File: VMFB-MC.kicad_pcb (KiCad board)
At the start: 2 copper layers, 64.6 x 67.3 mm, 45 parts, among them J1 Conn_01x04_Pin, J10 Conn_01x04_Pin, J2 Conn_01x04_Pin, J3 Conn_01x04_Pin, J4 Conn_01x02_Pin, J5 Conn_01x03_Pin, J6 Conn_01x04_Pin, J7 Conn_01x04_Pin, J8 Conn_01x04_Pin, J9 Conn_01x05_Pin, Q1 SFH313FA-2/3, Q2 SFH313FA-2/3, Q3 SFH313FA-2/3, Q4 SFH313FA-2/3, Q5 SFH313FA-2/3, Q6 SFH313FA-2/3, Q7 TIP120, Q8 TIP120, Q9 SFH313FA-2/3, U1 LM393

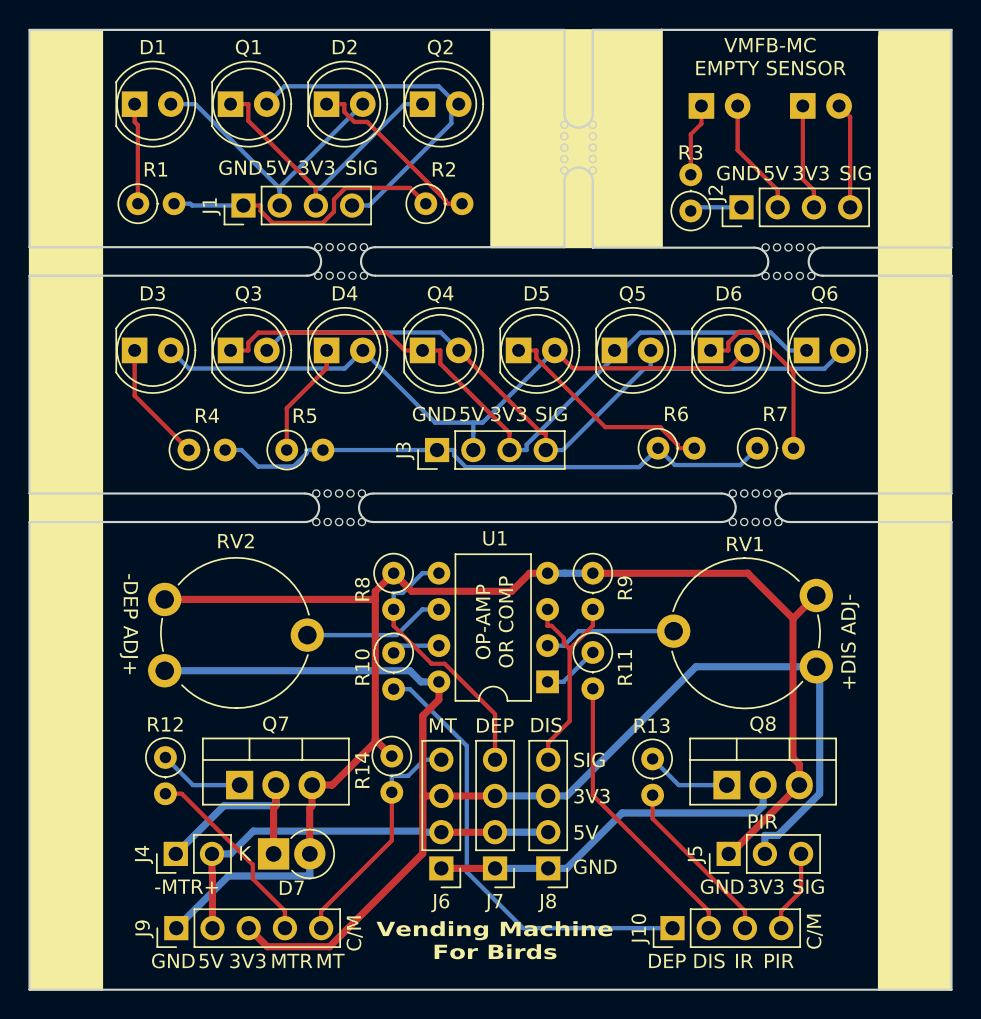
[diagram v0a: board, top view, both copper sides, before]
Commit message: more cleanup
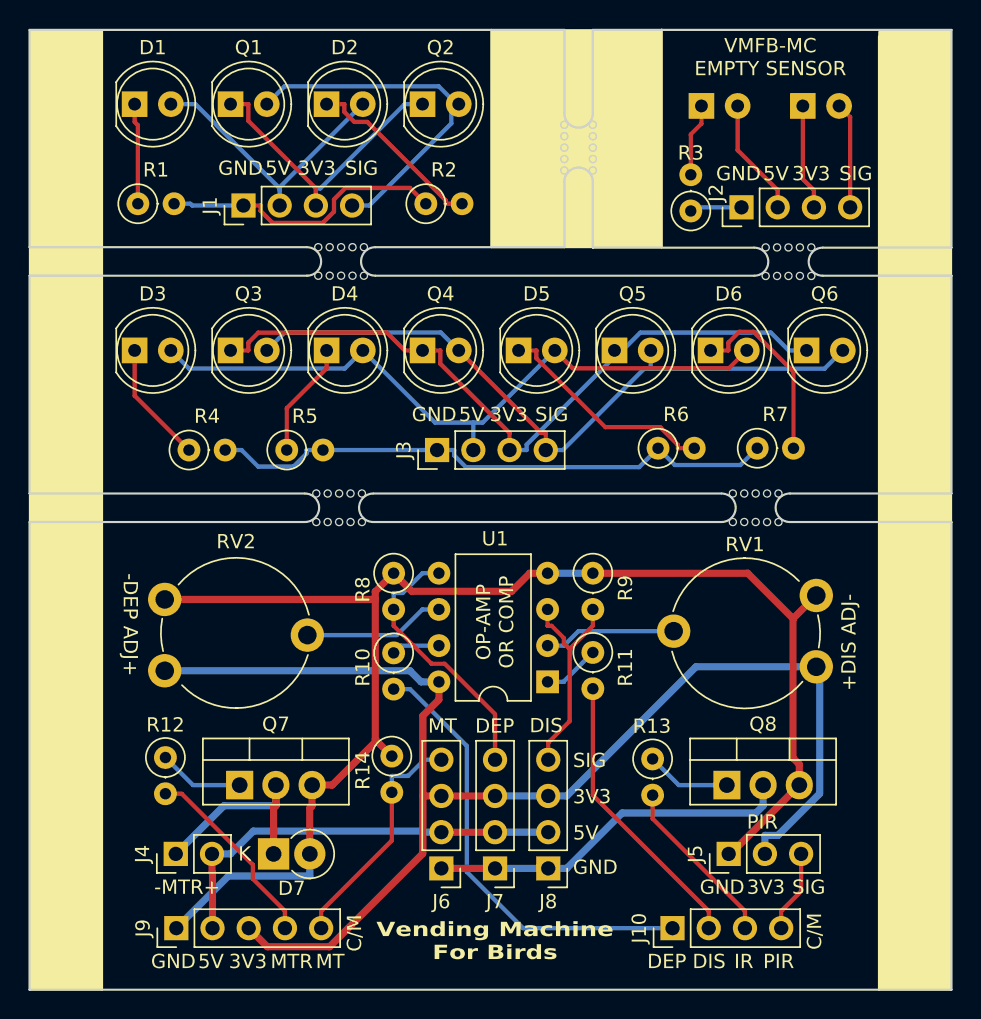
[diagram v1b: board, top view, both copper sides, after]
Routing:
- net Net-(J1-Pin_4): track 25.4 -> 24.5 mm
- net Net-(J3-Pin_3): track 50.6 -> 49.9 mm
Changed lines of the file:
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@@
   (segment (start 153.6182 101.1141) (end 153.6182 91.3248) (width 0.5) (layer "F.Cu") (net 2))
   (segment (start 133.8779 89.408) (end 126.873 89.408) (width 0.5) (layer "F.Cu") (net 2))
-  (segment (start 149.225 107.823) (end 149.098 107.823) (width 0.5) (layer "F.Cu") (net 2))
   (segment (start 154.051 101.5469) (end 153.6182 101.1141) (width 0.5) (layer "F.Cu") (net 2))
   (segment (start 119.888 104.4471) (end 119.726 104.6091) (width 0.5) (layer "F.Cu") (net 2))
@@
   (segment (start 119.726 107.823) (end 119.726 109.3731) (width 0.5) (layer "B.Cu") (net 2))
   (segment (start 114.0199 109.3731) (end 119.726 109.3731) (width 0.5) (layer "B.Cu") (net 2))
-  (segment (start 136.398 88.138) (end 137.6481 88.138) (width 0.5) (layer "B.Cu") (net 2))
+  (segment (start 136.398 88.138) (end 139.573 88.138) (width 0.5) (layer "B.Cu") (net 2))
   (segment (start 110.363 113.03) (end 114.0199 109.3731) (width 0.5) (layer "B.Cu") (net 2))
-  (segment (start 139.573 88.138) (end 137.6481 88.138) (width 0.5) (layer "B.Cu") (net 2))
   (segment (start 120.899 55.245) (end 122.1491 55.245) (width 0.3) (layer "F.Cu") (net 3))
   (segment (start 122.1491 55.792) (end 122.8522 56.4951) (width 0.3) (layer "F.Cu") (net 3))
@@
   (segment (start 132.715 103.759) (end 136.445 103.759) (width 0.5) (layer "B.Cu") (net 7))
   (segment (start 137.7451 103.759) (end 146.8021 94.702) (width 0.5) (layer "B.Cu") (net 7))
-  (segment (start 155.241 94.702) (end 155.478 94.939) (width 0.5) (layer "B.Cu") (net 7))
   (segment (start 151.638 107.823) (end 151.638 106.5229) (width 0.5) (layer "B.Cu") (net 7))
   (segment (start 155.478 103.6023) (end 152.5574 106.5229) (width 0.5) (layer "B.Cu") (net 7))
@@
   (segment (start 136.906 72.517) (end 138.1561 73.7671) (width 0.3) (layer "F.Cu") (net 24))
   (segment (start 149.1179 73.7671) (end 150.368 72.517) (width 0.3) (layer "F.Cu") (net 24))
-  (segment (start 131.191 78.3019) (end 131.191 77.5783) (width 0.3) (layer "B.Cu") (net 24))
+  (segment (start 131.191 79.502) (end 131.191 77.5783) (width 0.3) (layer "B.Cu") (net 24))
   (segment (start 122.1709 73.7901) (end 111.2551 73.7901) (width 0.3) (layer "B.Cu") (net 24))
   (segment (start 128.5053 77.5783) (end 131.191 77.5783) (width 0.3) (layer "B.Cu") (net 24))
   (segment (start 123.444 72.517) (end 122.1709 73.7901) (width 0.3) (layer "B.Cu") (net 24))
-  (segment (start 131.191 79.502) (end 131.191 78.3019) (width 0.3) (layer "B.Cu") (net 24))
   (segment (start 111.2551 73.7901) (end 109.982 72.517) (width 0.3) (layer "B.Cu") (net 24))
   (segment (start 123.444 72.517) (end 128.5053 77.5783) (width 0.3) (layer "B.Cu") (net 24))
@@
   (segment (start 129.6498 56.5993) (end 129.6498 55.245) (width 0.3) (layer "B.Cu") (net 29))
   (segment (start 123.8921 62.357) (end 129.6498 56.5993) (width 0.3) (layer "B.Cu") (net 29))
-  (segment (start 129.6498 55.245) (end 129.6498 54.8799) (width 0.3) (layer "B.Cu") (net 29))
   (segment (start 122.692 62.357) (end 123.8921 62.357) (width 0.3) (layer "B.Cu") (net 29))
-  (segment (start 130.17 55.245) (end 129.6498 55.245) (width 0.3) (layer "B.Cu") (net 29))
   (segment (start 129.6498 54.8799) (end 128.7647 53.9948) (width 0.3) (layer "B.Cu") (net 29))
   (segment (start 149.997 62.484) (end 146.695 62.484) (width 0.3) (layer "B.Cu") (net 30))
-  (segment (start 146.695 62.484) (end 146.441 62.738) (width 0.3) (layer "B.Cu") (net 30))
   (segment (start 154.3 55.372) (end 154.3 60.5069) (width 0.3) (layer "F.Cu") (net 31))
   (segment (start 155.077 62.484) (end 155.077 61.2839) (width 0.3) (layer "F.Cu") (net 31))
@@
   (segment (start 133.731 79.502) (end 133.731 78.3019) (width 0.3) (layer "F.Cu") (net 34))
   (segment (start 127.63 72.517) (end 126.3799 72.517) (width 0.3) (layer "F.Cu") (net 34))
-  (segment (start 141.092 72.517) (end 141.092 73.0799) (width 0.3) (layer "B.Cu") (net 34))
   (segment (start 152.0588 71.2669) (end 153.3089 72.517) (width 0.3) (layer "B.Cu") (net 34))
   (segment (start 134.9311 79.502) (end 134.9311 79.1234) (width 0.3) (layer "B.Cu") (net 34))
@@
   (segment (start 154.559 72.517) (end 153.3089 72.517) (width 0.3) (layer "B.Cu") (net 34))
   (segment (start 141.092 73.0799) (end 142.905 71.2669) (width 0.3) (layer "B.Cu") (net 34))
-  (segment (start 140.9746 73.0799) (end 141.092 73.0799) (width 0.3) (layer "B.Cu") (net 34))
   (segment (start 142.905 71.2669) (end 152.0588 71.2669) (width 0.3) (layer "B.Cu") (net 34))
   (segment (start 135.9549 78.3019) (end 130.17 72.517) (width 0.3) (layer "F.Cu") (net 35))
